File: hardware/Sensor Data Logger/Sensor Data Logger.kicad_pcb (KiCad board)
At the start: 2 copper layers, 131.3 x 62.5 mm, 76 parts, among them IC1 BQ25303JRTER, J1 Conn_01x04_Male, J2 Conn_01x04_Male, J3 Conn_01x05_Male, J4 Conn_01x03_Male, J5 MEM2051-00-195-00-A, J6 USB4055-30-A, M1 MountingHole_2.5mm_Pad, M2 MountingHole_2.5mm_Pad, M3 MountingHole_2.5mm_Pad, M4 MountingHole_2.5mm_Pad, Q1 Q_PMOS_DGS, Q2 NTJD1155LT2G, SW1 SW_Push, SW2 SW_Push, SW3 SW_Push, SW4 SW_SPDT, U1 AMS1117-3.3, U2 ESP32-WROOM-32, U3 DS3231M

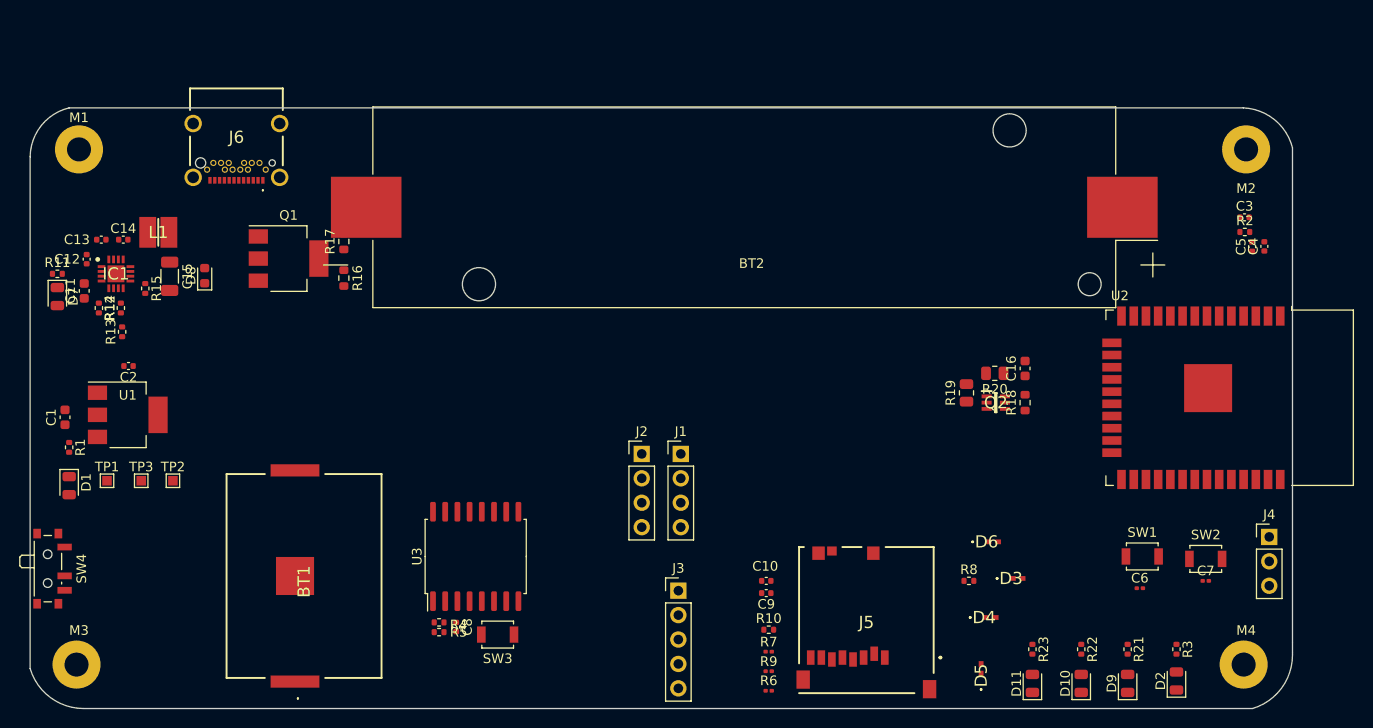
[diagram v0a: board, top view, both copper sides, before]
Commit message: Update latest hardware changes
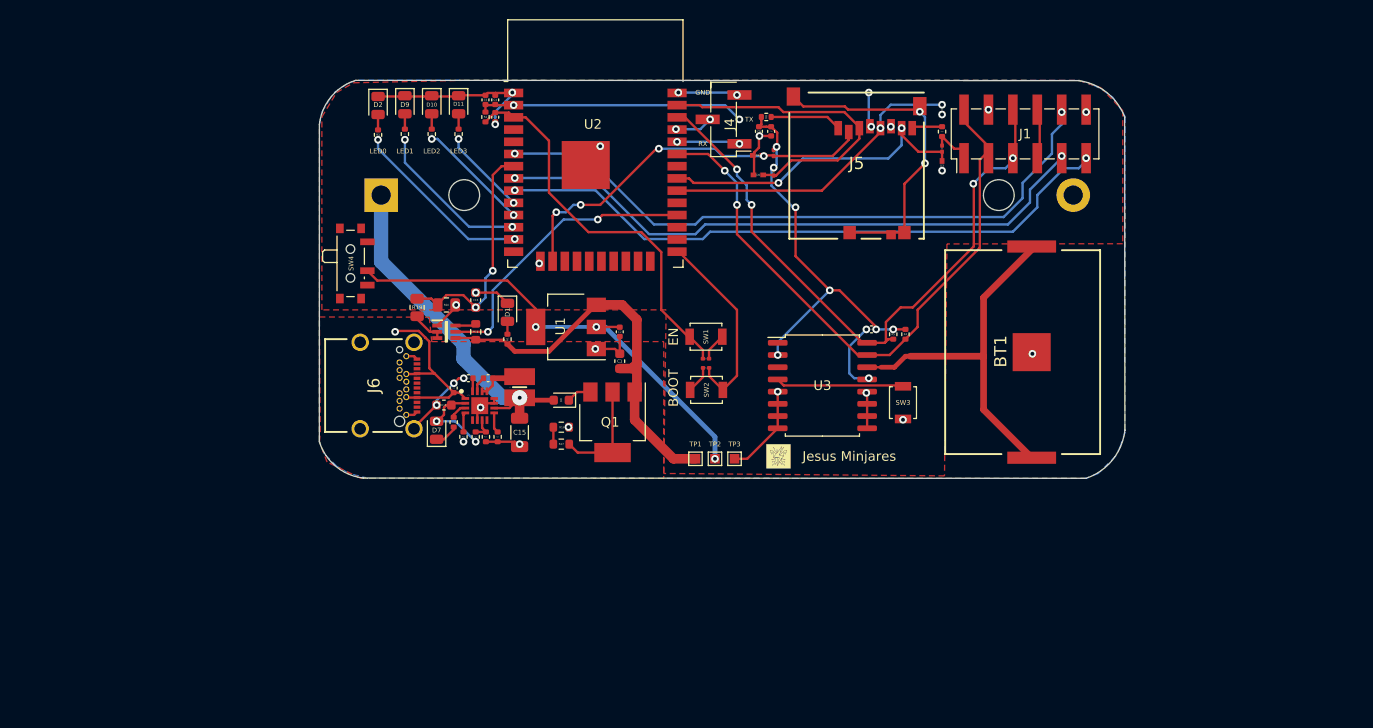
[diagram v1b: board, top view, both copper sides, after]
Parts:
- removed J2: Conn_01x04_Male, Connector_PinHeader_2.54mm:PinHeader_1x04_P2.54mm_Vertical
- removed J3: Conn_01x05_Male, Connector_PinHeader_2.54mm:PinHeader_1x05_P2.54mm_Vertical
- removed M1, M2, M3, M4: MountingHole_2.5mm_Pad, MountingHole:MountingHole_2.5mm_Pad
- added G***: LOGO, jminjares4 logo:jminjares4_small, F.Cu at (166.1, 95.5)
- added G***: LOGO, Github:github_small, B.Cu at (192.5, 93.7)
- added G***: LOGO, jminjares4 logo:jminjares4_tiny, B.Cu at (192.5, 88.1)
- BT2: footprint Battery:BatteryHolder_Keystone_1042_1x18650 -> Battery:BatteryHolder_MPD_BH-18650-PC2; moved to B.Cu
- J1: value Conn_01x04_Male -> Conn_01x12_Male; footprint Connector_PinHeader_2.54mm:PinHeader_1x04_P2.54mm_Vertical -> Connector_PinHeader_2.54mm:PinHeader_2x06_P2.54mm_Vertical_SMD
- J4: footprint Connector_PinHeader_2.54mm:PinHeader_1x03_P2.54mm_Vertical -> Connector_PinHeader_2.54mm:PinHeader_1x03_P2.54mm_Vertical_SMD_Pin1Left
- moved D2 102.4 mm to (124.5, 59.0), turned to -90 degrees
- moved R3 98.8 mm to (124.5, 62.1), turned to 90 degrees
- moved D9 96.3 mm to (127.3, 58.9), turned to -90 degrees
- moved R21 92.3 mm to (127.3, 62.0), turned to 90 degrees
- moved D10 90.5 mm to (130.0, 58.9), turned to -90 degrees
- moved R22 86.2 mm to (130.0, 62.0), turned to 90 degrees
- moved D11 84.8 mm to (132.8, 58.9), turned to -90 degrees
- moved C4 81.4 mm to (136.7, 58.4)
- moved C5 81.2 mm to (135.6, 58.4)
- moved R23 80.2 mm to (132.8, 62.0), turned to 90 degrees
- moved BT1 80.1 mm to (192.5, 84.7), turned to 90 degrees
- moved R2 79.9 mm to (135.6, 60.2), turned to 90 degrees
- moved C3 78.6 mm to (136.7, 60.2), turned to -90 degrees
- moved J4 71.5 mm to (160.4, 60.5), turned to 180 degrees
- moved U2 67.2 mm to (147.1, 66.0), turned to 0 degrees
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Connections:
- BT1 pad 2: GND -> Net-(BT1-Pad1)
- BT1 pad 3: (no net) -> GND
- J1 pad 3: /SCL -> /SDA
- SW4 pad 1: unconnected-(SW4-Pad1) -> VCC
- SW4 pad 3: VCC -> unconnected-(SW4-Pad3)
- U2 pad 10: /LED_1 -> /LED_3
- U2 pad 12: /LED_3 -> /LED_1
- U2 pad 13: unconnected-(U2-Pad13) -> /LED_0
- U2 pad 16: /SD_CLK -> /SD_CS
- U2 pad 24: /LED_0 -> unconnected-(U2-Pad24)
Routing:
- net VCC: track 0.00 -> 80.1 mm, vias 0 -> 11
- net GND: track 0.00 -> 80.0 mm, vias 0 -> 28
- net /A2: track 0.00 -> 67.6 mm, vias 0 -> 2
- net /A1: track 0.00 -> 65.9 mm, vias 0 -> 2
- net /SCL: track 0.00 -> 64.5 mm, vias 0 -> 4
- net /A0: track 0.00 -> 63.7 mm, vias 0 -> 2
- net /SDA: track 0.00 -> 63.3 mm, vias 0 -> 2
- net Net-(C2-Pad1): track 0.00 -> 49.2 mm, vias 0 -> 3
- net +BATT: track 0.00 -> 42.6 mm
- net /EN: track 0.00 -> 40.8 mm
- net /BAT: track 0.00 -> 40.6 mm, vias 0 -> 1
- net /SD_CS: track 0.00 -> 40.3 mm, vias 0 -> 4
- net Net-(BT1-Pad1): track 0.00 -> 38.7 mm
- net /SD_MISO: track 0.00 -> 33.9 mm, vias 0 -> 2
- net Net-(J5-PadMP1): track 0.00 -> 33.5 mm, vias 0 -> 2
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- added copper zone on B.Cu, net GND
- added copper zone on F.Cu, net VBUS
- added copper zone on F.Cu, net VCC
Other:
- board size 131.3 x 62.5 mm -> 83.8 x 41.4 mm
- board text added: "+"
- board text added: "BOOT"
- board text added: "EN"
- board text added: "GND"
- board text added: "Jesus Minjares"
- board text added: "LED0"
- board text added: "LED1"
- board text added: "LED2"
- board text added: "LED3"
- board text added: "RX"
- board text added: "TX"
- board text added: "jminjares4"
